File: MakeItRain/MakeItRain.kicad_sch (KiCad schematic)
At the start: 26 parts, among them IC1 OPA2340PA, IC2 LM2597MX-5.0_NOPB, J1 Conn_02x16_Odd_Even, J2 Conn_02x19_Odd_Even, J3 Conn_01x19, P1 Screw_Terminal_01x02, Q1 IRF9Z34NPBF, U1 178.6165.0001

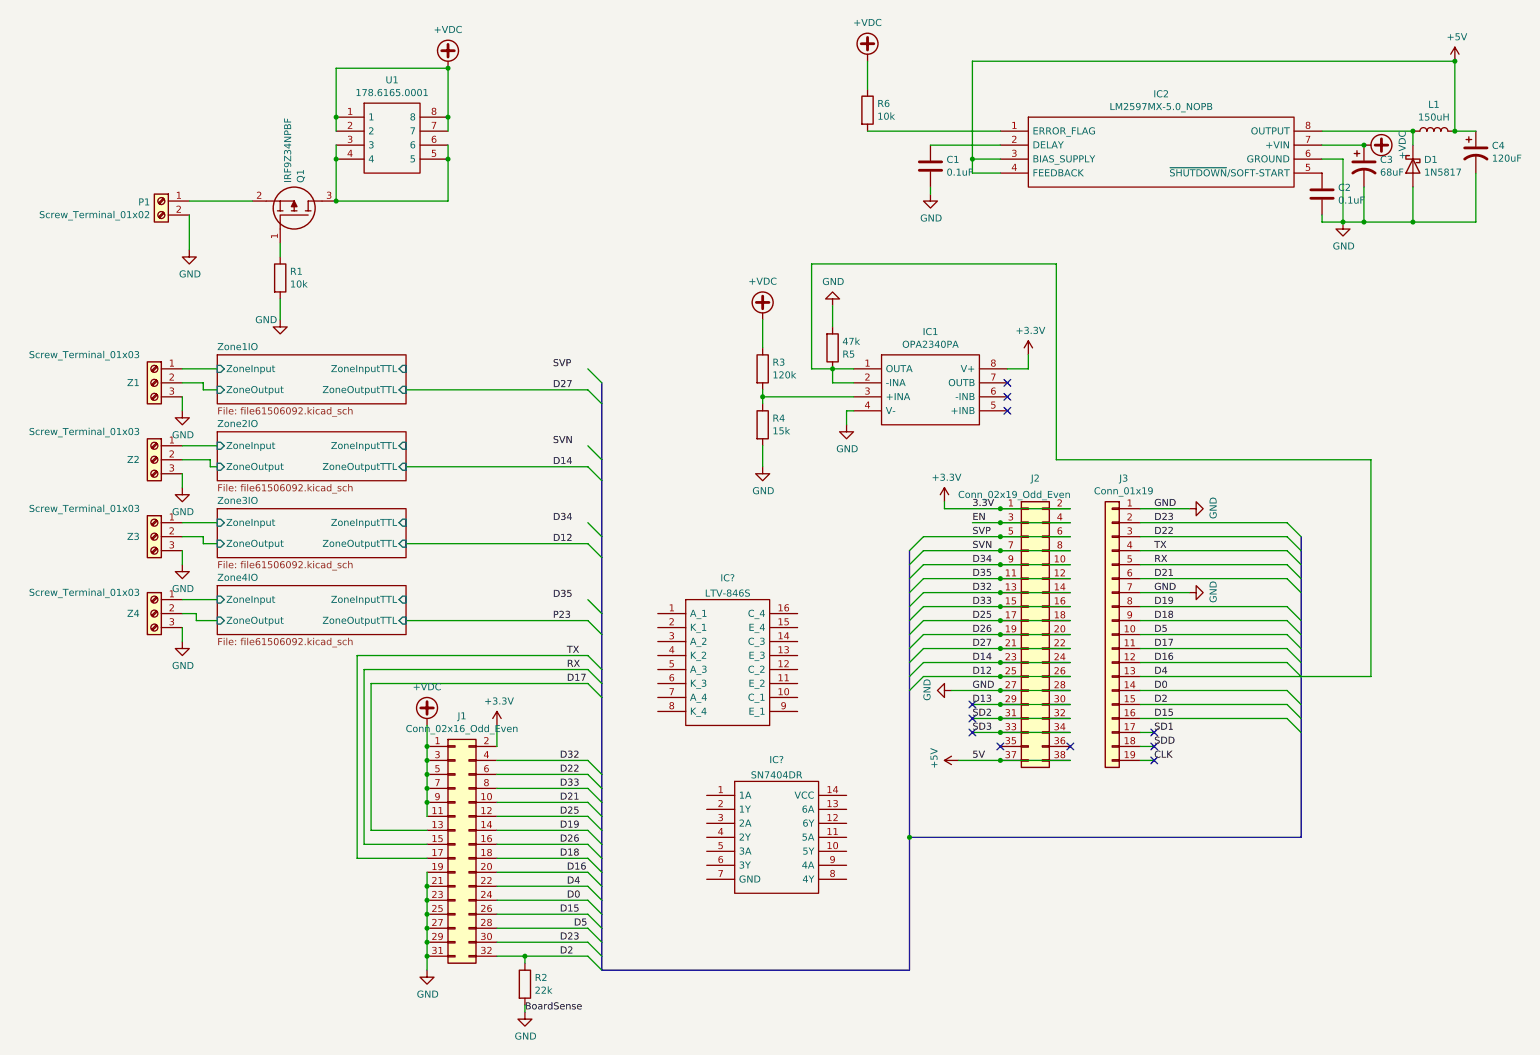
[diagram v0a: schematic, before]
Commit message: wip for hardware
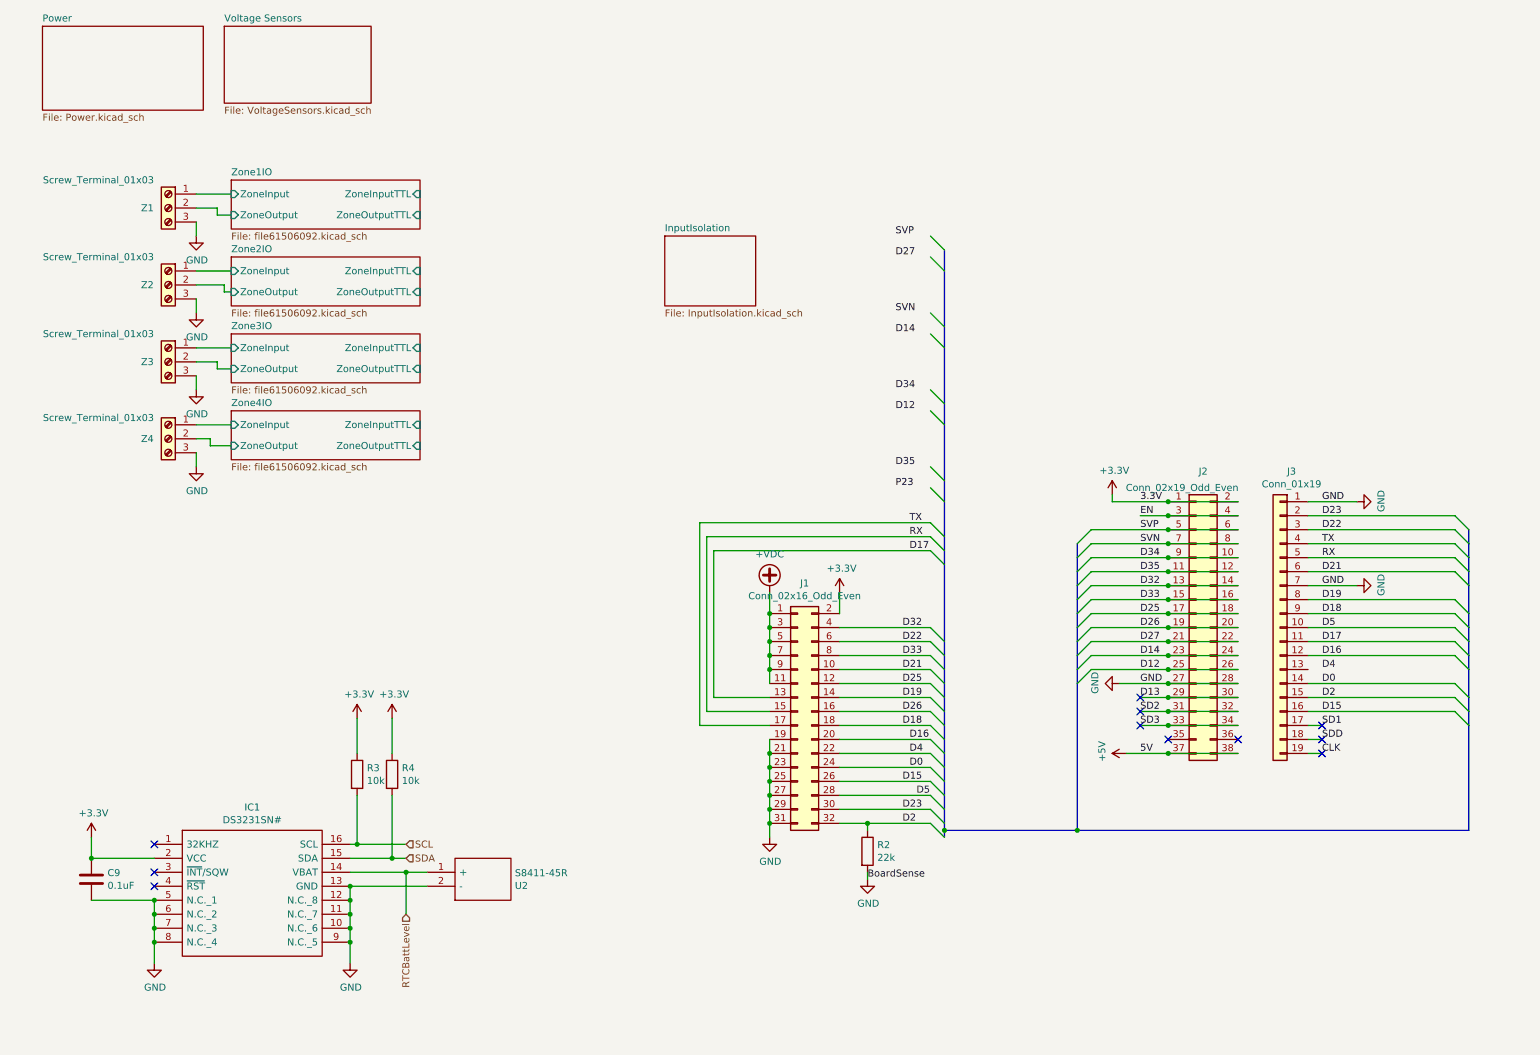
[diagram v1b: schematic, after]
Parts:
- removed C1, C2: 0.1uF, Capacitor_THT:C_Disc_D4.7mm_W2.5mm_P5.00mm, symbol Device:C
- removed C3: 68uF, Capacitor_THT:CP_Radial_D8.0mm_P3.50mm, symbol Device:CP1
- removed C4: 120uF, Capacitor_THT:CP_Radial_D8.0mm_P3.50mm, symbol Device:CP1
- removed D1: 1N5817, Diode_THT:D_DO-41_SOD81_P10.16mm_Horizontal, symbol Diode:1N5817
- removed IC1: OPA2340PA, SamacSys_Parts:DIP794W53P254L959H508Q8N, symbol SamacSys_Parts:OPA2340PA
- removed IC2: LM2597MX-5.0_NOPB, SamacSys_Parts:SOIC127P600X175-8N, symbol SamacSys_Parts:LM2597MX-5.0_NOPB
- removed IC?: LTV-846S, SOP254P1016X460-16N, symbol Samac_Sys:LTV-846S
- removed IC?: SN7404DR, SOIC127P600X175-14N, symbol Samac_Sys:SN7404DR
- removed L1: 150uH, Inductor_THT:L_Axial_L6.6mm_D2.7mm_P10.16mm_Horizontal_Vishay_IM-2, symbol Device:L
- removed P1: Screw_Terminal_01x02, TerminalBlock_Phoenix:TerminalBlock_Phoenix_MKDS-1,5-2-5.08_1x02_P5.08mm_Horizontal, symbol Connector:Screw_Terminal_01x02
- removed Q1: IRF9Z34NPBF, SamacSys_Parts:TO254P469X1042X1967-3P, symbol SamacSys_Parts:IRF9Z34NPBF
- removed R1, R6: 10k, Resistor_THT:R_Axial_DIN0207_L6.3mm_D2.5mm_P5.08mm_Vertical, symbol Device:R
- removed R5: 47k, Resistor_THT:R_Axial_DIN0207_L6.3mm_D2.5mm_P5.08mm_Vertical, symbol Device:R
- removed U1: 178.6165.0001, SamacSys_Parts:17861650001, symbol SamacSys_Parts:178.6165.0001
- added C9: 0.1uF, Capacitor_THT:C_Rect_L9.0mm_W3.6mm_P7.50mm_MKT, symbol Device:C
- added IC1: DS3231SN#, SamacSys_Parts:SOIC127P1032X265-16N, symbol SamacSys_Parts:DS3231SN#
- added U2: S8411-45R, SamacSys_Parts:S8411-45R_1, symbol SamacSys_Parts:S8411-45R
- R3: value 120k -> 10k; footprint Resistor_THT:R_Axial_DIN0207_L6.3mm_D2.5mm_P5.08mm_Vertical -> Resistor_THT:R_Axial_DIN0207_L6.3mm_D2.5mm_P2.54mm_Vertical
- R4: value 15k -> 10k; footprint Resistor_THT:R_Axial_DIN0207_L6.3mm_D2.5mm_P5.08mm_Vertical -> Resistor_THT:R_Axial_DIN0207_L6.3mm_D2.5mm_P2.54mm_Vertical
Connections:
- net +3V3: now also R3.1, R4.1, C9.1, IC1.2 (VCC)
- net +VDC: no longer R3.1
- net D4: no longer J3.13 (Pin_13)
- net GND: now also C9.2, IC1.10 (N.C._6), IC1.11 (N.C._7), IC1.12 (N.C._8), IC1.13 (GND), IC1.5 (N.C._1), IC1.6 (N.C._2), IC1.7 (N.C._3), IC1.8 (N.C._4), IC1.9 (N.C._5), U2.2 (-); no longer R4.2
- net SCL: now reaches R3.2
- net SCL: now also IC1.16 (SCL); no longer R4.1
- new net RTCBattLevel: IC1.14 (VBAT), U2.1 (+)
- new net SDA: IC1.15 (SDA), R4.2
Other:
- added sheet InputIsolation (InputIsolation.kicad_sch)
- added sheet Power (Power.kicad_sch)
- added sheet Voltage Sensors (VoltageSensors.kicad_sch)
- moved on the sheet: J1, J2, J3, R2, Z1, Z2, Z3, Z4
